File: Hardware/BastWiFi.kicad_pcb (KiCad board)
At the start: 2 copper layers, 60 x 22.9 mm, 31 parts, among them J1 Conn_Battery, J2 USB_B_Micro, J3 Conn_Left, J4 Conn_Right, Q1 DMG3415U-7, SW1 GPIO0, SW2 RESET, U1 MCP73831-3-OT, U2 AP2112K-3.3, U3 ESP32-S2-WROVER

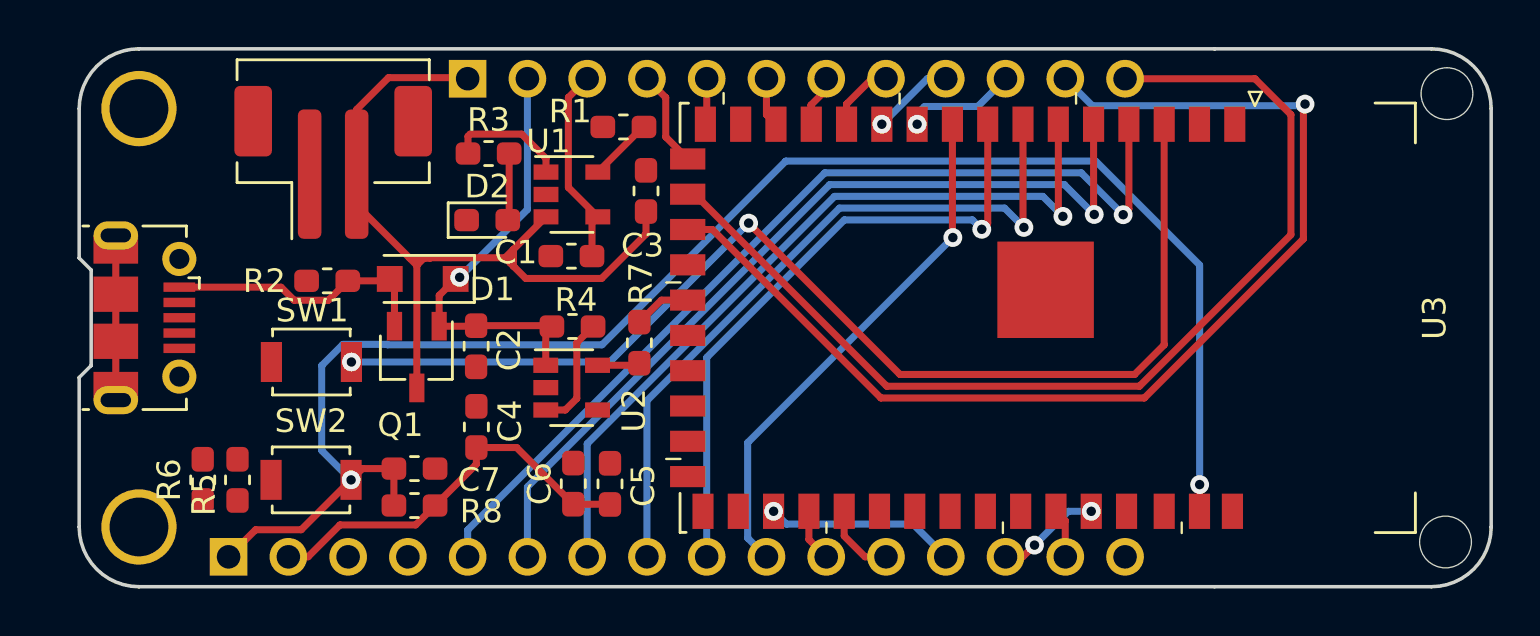
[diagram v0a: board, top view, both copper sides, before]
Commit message: Add connector
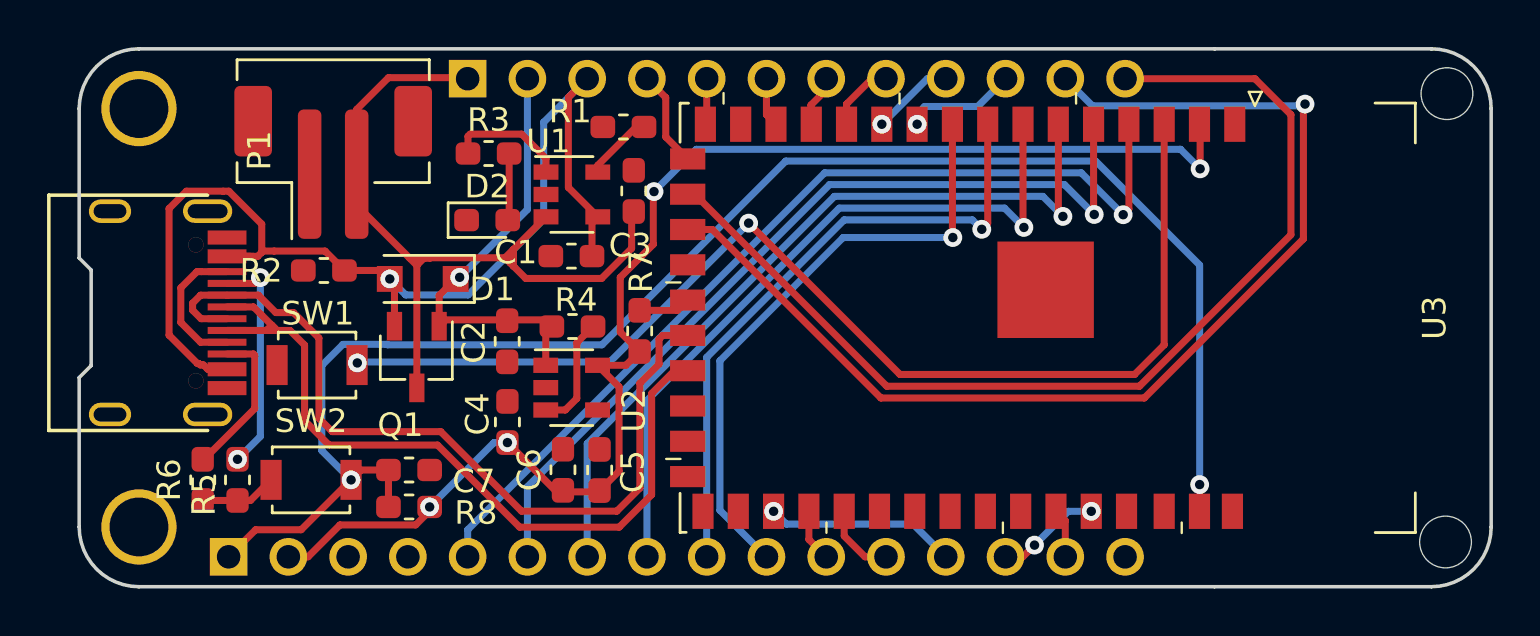
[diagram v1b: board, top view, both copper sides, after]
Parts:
- removed J2: USB_B_Micro, Connector_USB:USB_Micro-B_Molex-105017-0001
- added P1: USB_C_Plug_USB2.0, Connectors EC:C393939, F.Cu at (132.5, 92.5)
- moved C2 1.34 mm to (145.2, 93.7)
- moved C4 1.34 mm to (145.2, 97.1)
- moved C6 0.74 mm to (147.6, 99.2)
- moved C5 0.74 mm to (149.1, 99.2)
- moved C3 0.52 mm to (150.6, 87.3)
- moved R7 0.50 mm to (150.8, 93.3)
- moved R2 0.46 mm to (137.4, 90.7)
- moved SW1 0.27 mm to (137.1, 94.7)
- moved C7 0.24 mm to (141.0, 99.2)
- moved R8 0.24 mm to (141.0, 100.8)
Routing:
- net +3V3: track 18.8 -> 58.2 mm, vias 0 -> 4
- net /D-: track 0.00 -> 35.2 mm
- net /D+: track 0.00 -> 34.9 mm
- net VBUS: track 20.1 -> 49.6 mm, vias 0 -> 1
- net Net-(P1-PadA5): track 0.00 -> 9.64 mm, vias 0 -> 2
- net Net-(P1-PadB5): track 0.00 -> 6.57 mm
- net (no net): track 0.00 -> 6.04 mm
- net /A5: track 22.3 -> 26.0 mm
- net GND: track 5.80 -> 3.27 mm
